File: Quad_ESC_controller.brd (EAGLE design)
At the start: 25.4 x 38.1 mm, 36 parts, among them IC1 OP-AMP, Y1 ECS-80-S-4X

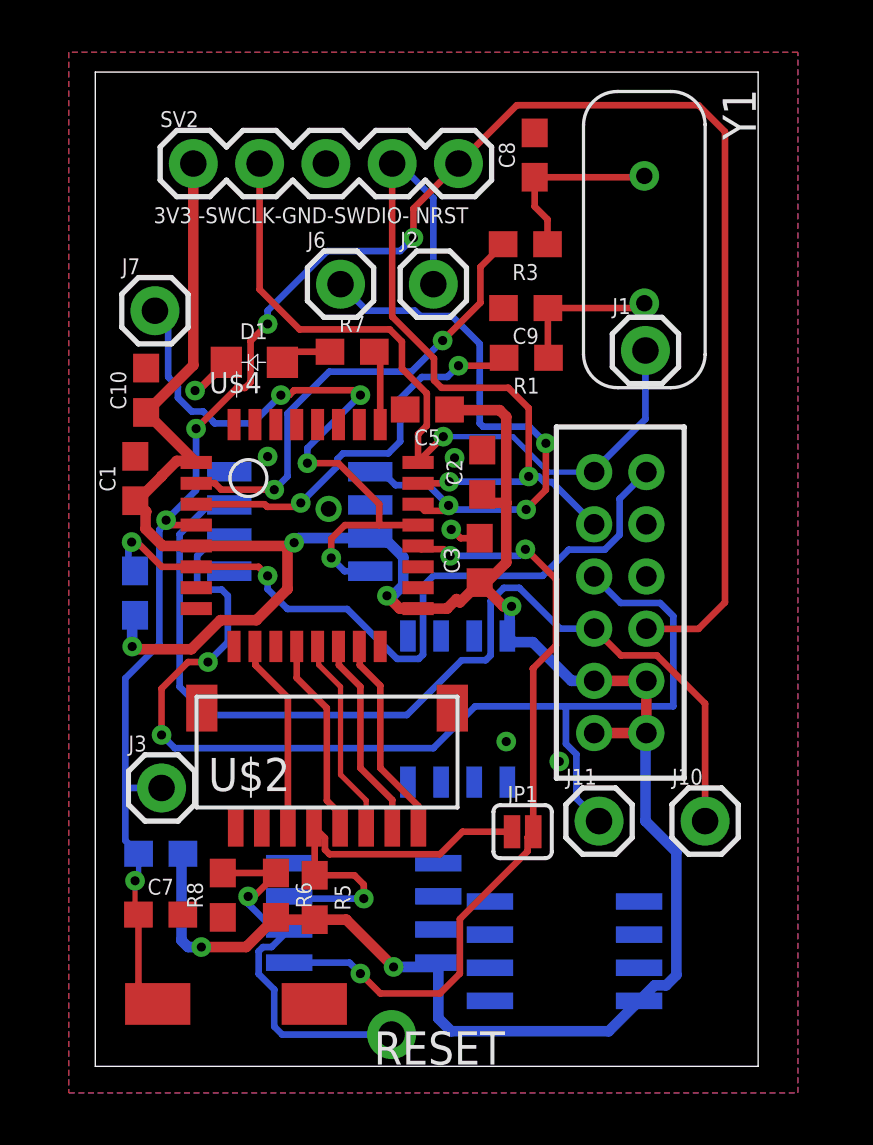
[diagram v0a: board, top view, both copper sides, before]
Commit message: check this
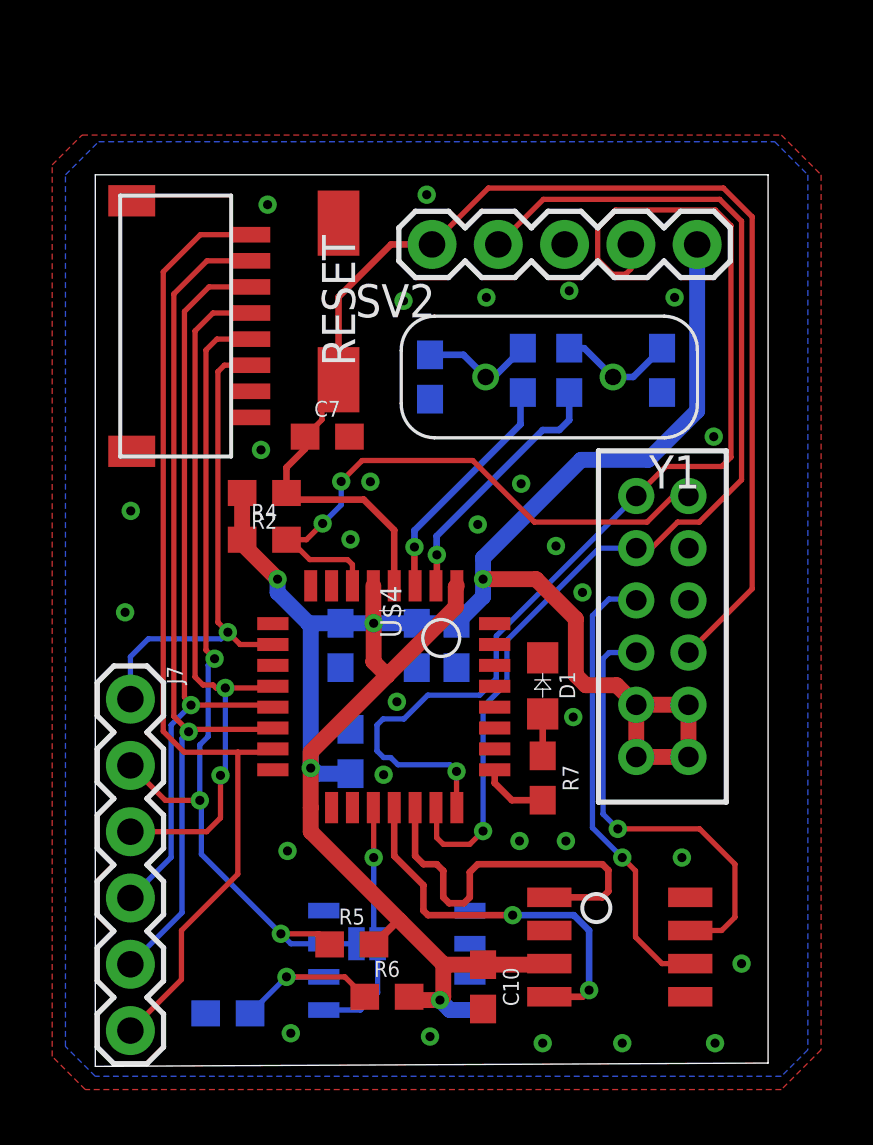
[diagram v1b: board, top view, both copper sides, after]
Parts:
- removed J1, J10, J11, J2, J3, J6, J8: (no value), SparkFun-Connectors:1X01
- removed OP-AMP, OP-AMP1: LM2904S, IC, LM2904:SO08
- J7: device SparkFun-Connectors:1X01 -> SparkFun-Connectors:1X06
- moved RESET 27.2 mm to (9.32, 29.3), turned to 270 degrees
- moved C10 26.3 mm to (14.9, 3.05), turned to 270 degrees
- moved SV2 19.6 mm to (23.1, 31.5), turned to 180 degrees
- moved C7 19.4 mm to (8.89, 24.1)
- moved R7 17.9 mm to (17.1, 11.0), turned to 270 degrees
- moved U$8 17.7 mm to (17.4, 2.67), flipped to the top
- moved D1 16.6 mm to (17.1, 14.6), turned to 270 degrees
- moved J7 14.9 mm to (1.35, 14.1), turned to 270 degrees
- moved R2 14.4 mm to (6.48, 22.0), flipped to the top
- moved C1 13.9 mm to (13.8, 16.1), flipped to the bottom, turned to 270 degrees
- moved U$2 13.5 mm to (5.21, 23.4), turned to 90 degrees
- moved C2 11.8 mm to (9.78, 12.1), flipped to the bottom
- moved IC1 9.91 mm to (11.6, 4.06), turned to 90 degrees
- moved C5 9.64 mm to (9.40, 16.1), flipped to the bottom, turned to 270 degrees
- moved C8 9.58 mm to (21.7, 26.7), flipped to the bottom, turned to 270 degrees
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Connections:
- net +3V3: no longer OP-AMP.8, OP-AMP1.8
- net ADC: now also J7.1
- net CAN_H: no longer J10.1
- net CAN_L: no longer J11.1
- net CAN_RX: no longer J7.1
- net CAN_TX: no longer J6.1
- net GND: no longer OP-AMP.4, OP-AMP1.4
- net N$6: now also IC1.2; no longer J8.1, OP-AMP1.2
- net NRST: no longer J3.1
- net SWCLK: no longer J1.1
- net SWDIO: no longer J2.1
- net TIM3_CH1: now also J7.3
- net TIM3_CH2: now also J7.4
- net TIM3_CH3: now also J7.5
- net TIM3_CH4: now also J7.6
- net TLM: now also IC1.1; no longer OP-AMP1.1
- net TLM_ESC: now also IC1.3, J7.2; no longer OP-AMP1.3
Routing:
- net TIM3_CH4: track 7.86 -> 38.5 mm
- net CAN_L: track 43.8 -> 17.5 mm, vias 2 -> 1
- net TIM3_CH3: track 7.78 -> 33.6 mm, vias 0 -> 1
- net NRST: track 75.6 -> 50.9 mm, vias 5 -> 0
- net TIM3_CH2: track 7.69 -> 29.6 mm, vias 0 -> 1
- net CAN_H: track 38.4 -> 17.1 mm, vias 0 -> 1
- net TLM: track 30.0 -> 9.50 mm, vias 3 -> 1
- net TIM3_CH1: track 7.61 -> 27.6 mm, vias 0 -> 2
- net TLM_ESC: track 16.0 -> 34.2 mm, vias 1 -> 3
- net +3V3: track 103.6 -> 87.9 mm, vias 6 -> 5
- net SWDIO: track 28.7 -> 42.8 mm, vias 2 -> 1
- net SWCLK: track 29.5 -> 42.8 mm
- net ADC: track 7.45 -> 19.2 mm, vias 0 -> 1
- net CAN_RX: track 25.4 -> 15.0 mm, vias 4 -> 2
- net N$6: track 15.0 -> 6.72 mm
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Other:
- board size 25.4 x 38.1 mm -> 25.8 x 34.2 mm
- board text added: "C:/Users/Rach s PC/Desktop/kingsman logo.bmp'"
